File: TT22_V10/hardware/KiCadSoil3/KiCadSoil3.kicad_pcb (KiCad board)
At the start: 2 copper layers, 55.9 x 19.1 mm, 11 parts, among them J1 Screw_Terminal_01x03, J2 Conn_Coaxial, U1 ATtiny85-20PU, U2 TLC555CP

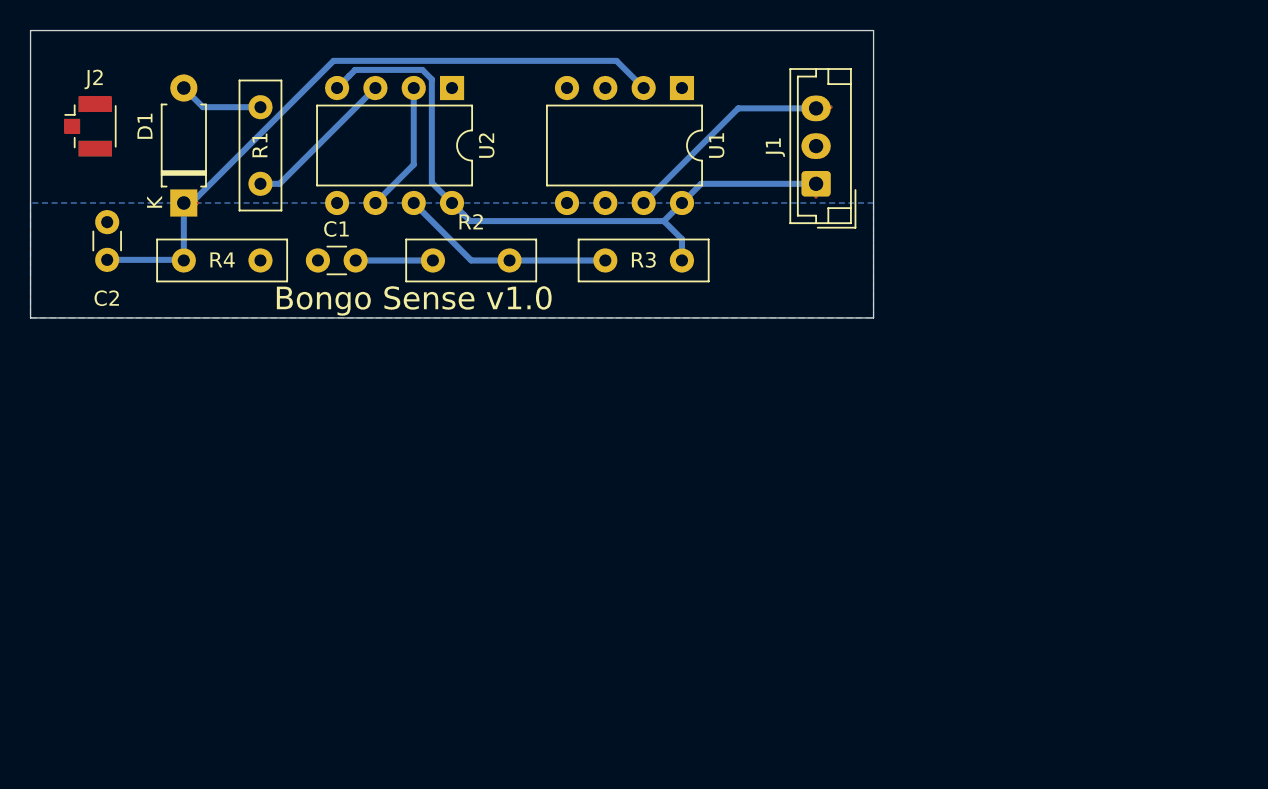
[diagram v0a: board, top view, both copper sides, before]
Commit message: drill
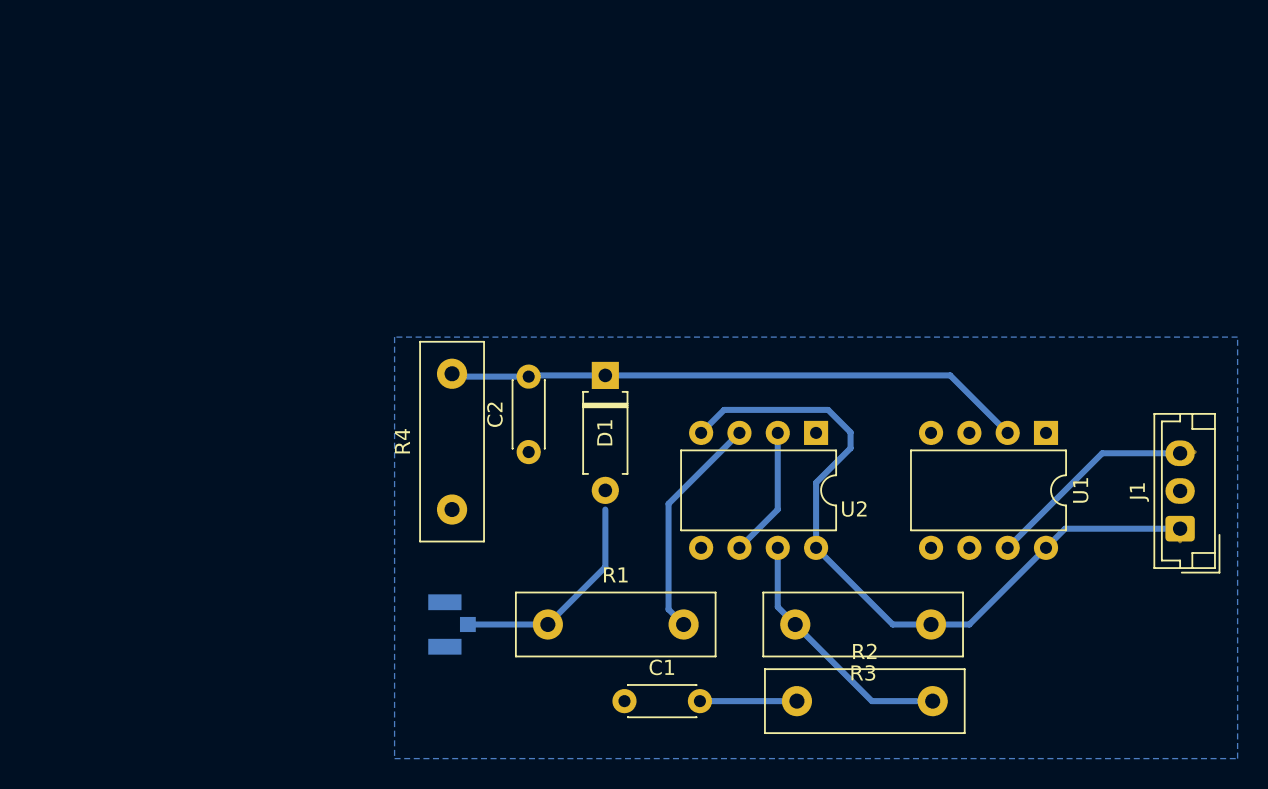
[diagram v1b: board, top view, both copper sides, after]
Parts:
- C1, C2: footprint Capacitor_THT:C_Disc_D3.0mm_W1.6mm_P2.50mm -> Capacitor_THT:C_Disc_D4.3mm_W1.9mm_P5.00mm
- J2: moved to B.Cu
- R1, R2, R3, R4: footprint Resistor_THT:R_Box_L8.4mm_W2.5mm_P5.08mm -> Resistor_THT:R_Box_L13.0mm_W4.0mm_P9.00mm
- moved J2 40.9 mm to (40.6, 52.1), turned to 180 degrees
- moved R1 39.2 mm to (47.0, 52.1), turned to 0 degrees
- moved R2 37.9 mm to (63.5, 57.1)
- moved C1 35.6 mm to (52.1, 57.1)
- moved J1 33.2 mm to (88.9, 45.7)
- moved U1 33.2 mm to (80.0, 39.4)
- moved U2 33.2 mm to (64.8, 39.4)
- moved C2 31.8 mm to (45.7, 40.6), turned to 90 degrees
- moved D1 30.2 mm to (50.8, 35.6), turned to 270 degrees
- moved R3 29.2 mm to (72.4, 52.1)
- moved R4 20.8 mm to (40.6, 44.5), turned to 90 degrees
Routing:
- net Net-(D1-Pad2): track 5.61 -> 14.5 mm
- net /AOUT: track 45.7 -> 38.5 mm
- net Net-(R1-Pad2): track 10.3 -> 15.1 mm
- net +3V3: track 45.4 -> 49.5 mm
- net Net-(R2-Pad2): track 14.3 -> 16.8 mm
- net Net-(C1-Pad2): track 5.12 -> 6.43 mm
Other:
- board outline removed
- board text removed: "Bongo Sense v1.0"

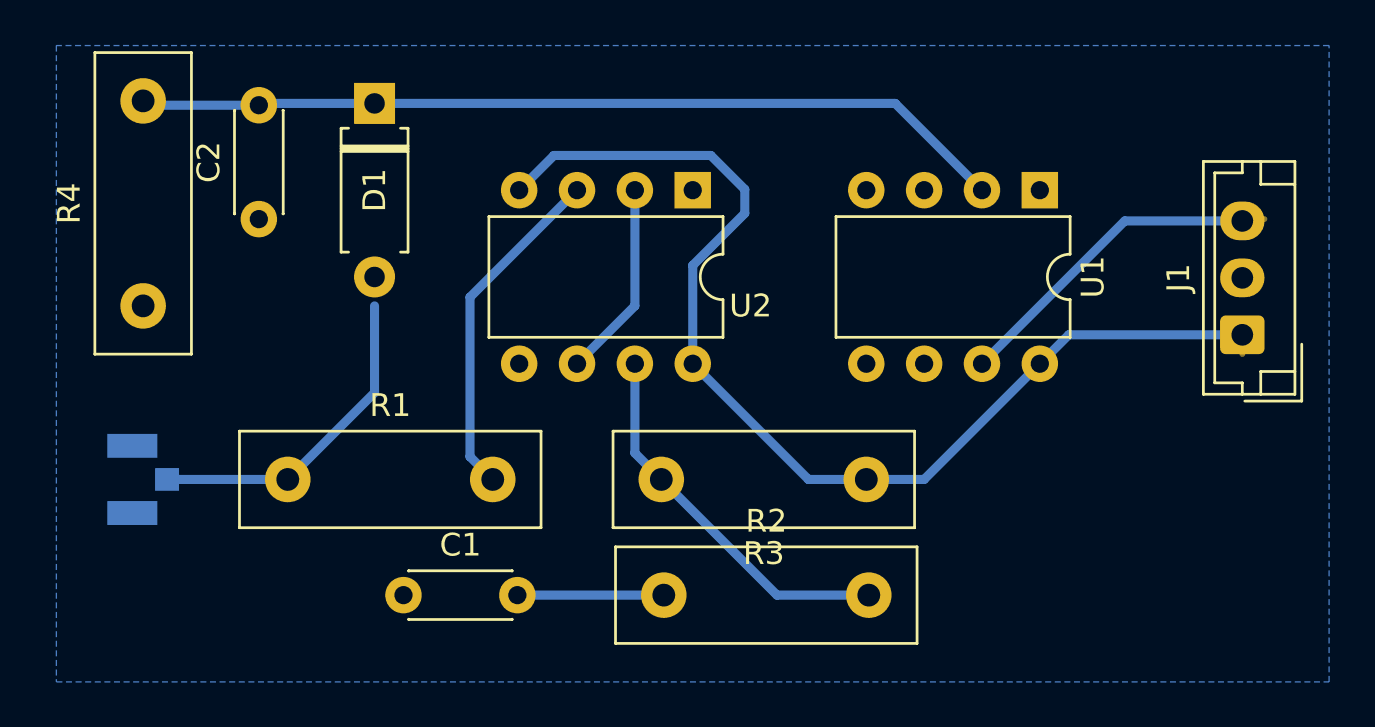
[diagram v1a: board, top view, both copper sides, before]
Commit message: changes
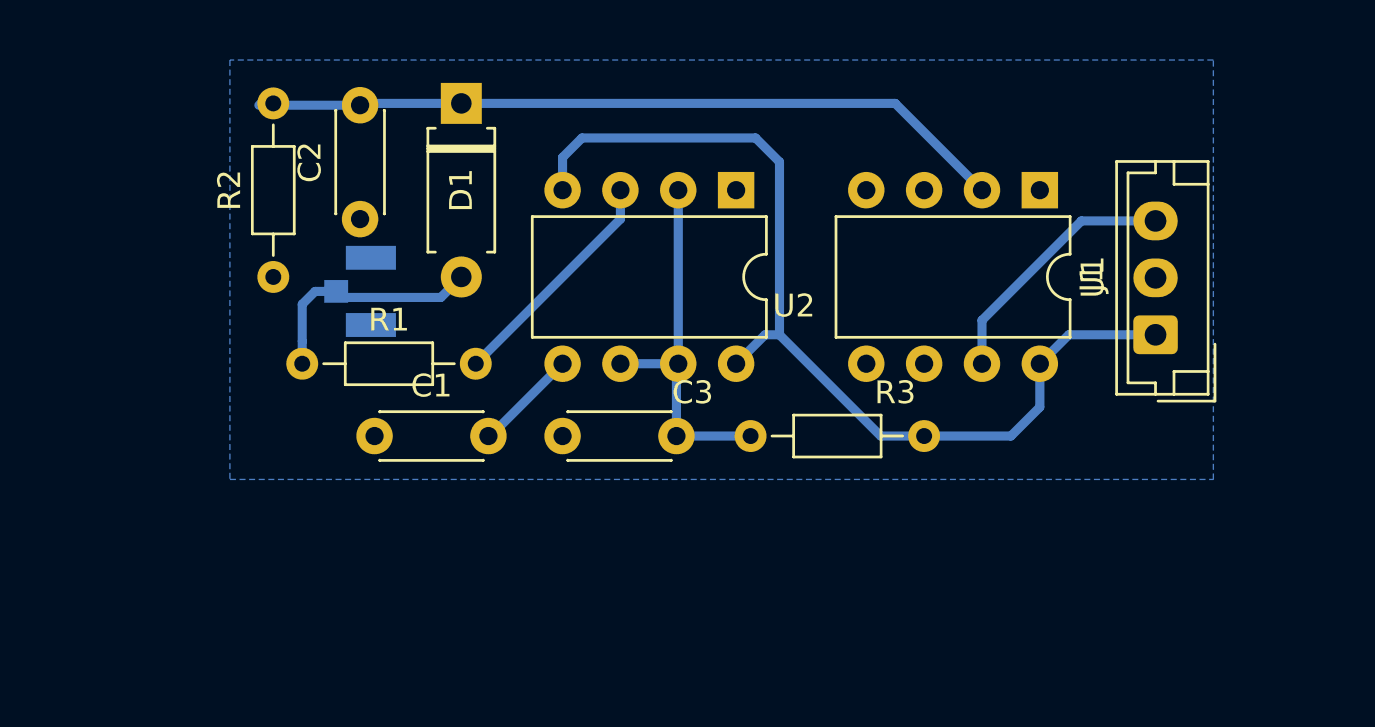
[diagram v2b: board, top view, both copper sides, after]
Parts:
- removed the R2 at (63.5, 57.1)
- added C3: 330p, Capacitor_THT:C_Disc_D4.3mm_W1.9mm_P5.00mm, F.Cu at (59.1, 50.2)
- C1: value 660p -> 10p
- C2: value 660p -> 1n
- R1, R3: footprint Resistor_THT:R_Box_L13.0mm_W4.0mm_P9.00mm -> Resistor_THT:R_Axial_DIN0204_L3.6mm_D1.6mm_P7.62mm_Horizontal
- R2: renamed from R4; footprint Resistor_THT:R_Box_L13.0mm_W4.0mm_P9.00mm -> Resistor_THT:R_Axial_DIN0204_L3.6mm_D1.6mm_P7.62mm_Horizontal
- moved J2 12.6 mm to (50.2, 43.8), turned to 0 degrees
- moved C1 7.10 mm to (50.8, 50.2)
- moved R2 5.85 mm to (46.4, 43.2)
- moved R1 5.12 mm to (47.6, 47.0)
- moved C2 4.45 mm to (50.2, 40.6)
- moved D1 3.81 mm to (54.6, 35.6)
- moved J1 3.81 mm to (85.1, 45.7)
- moved R3 3.18 mm to (74.9, 50.2)
- moved U2 1.91 mm to (66.7, 39.4)
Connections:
- R3 pad 2: Net-(R2-Pad2) -> Net-(C3-Pad2)
- U1 pad 1: (no net) -> GND
- U1 pad 3: (no net) -> GND
- U1 pad 5: (no net) -> GND
- U1 pad 6: (no net) -> GND
- U2 pad 2: Net-(U2-Pad2) -> Net-(C3-Pad2)
- U2 pad 5: GND -> Net-(C1-Pad2)
- U2 pad 6: Net-(U2-Pad2) -> Net-(C3-Pad2)
- U2 pad 7: Net-(R2-Pad2) -> Net-(C3-Pad2)
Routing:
- net Net-(R2-Pad2): track 16.8 -> 0.00 mm
- net Net-(C3-Pad2): track 0.00 -> 16.7 mm
- net Net-(U2-Pad2): track 8.67 -> 0.00 mm
- net +3V3: track 49.5 -> 43.1 mm
- net /AOUT: track 38.5 -> 32.9 mm
- net Net-(R1-Pad2): track 15.1 -> 10.3 mm
- net Net-(D1-Pad2): track 14.5 -> 10.3 mm
- net /1-Wire: track 15.0 -> 11.3 mm
- net Net-(C1-Pad2): track 6.43 -> 4.58 mm
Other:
- net class Default: clearance 0.2 -> 0.24
- net class Ground: clearance 0.2 -> 0.24
- rule trace_clearance: 0.2 -> 0.24
